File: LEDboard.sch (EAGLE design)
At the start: 312 parts, among them IC1 REG1117, Q1 MMUN2133LT1G, U1 IS31FL3741_QFN60, U2 IS31FL3741_QFN60, U3 ATSAMD21G-A, U4 TPS61090RSAR, U5 MCP73831T-2ACI/OT

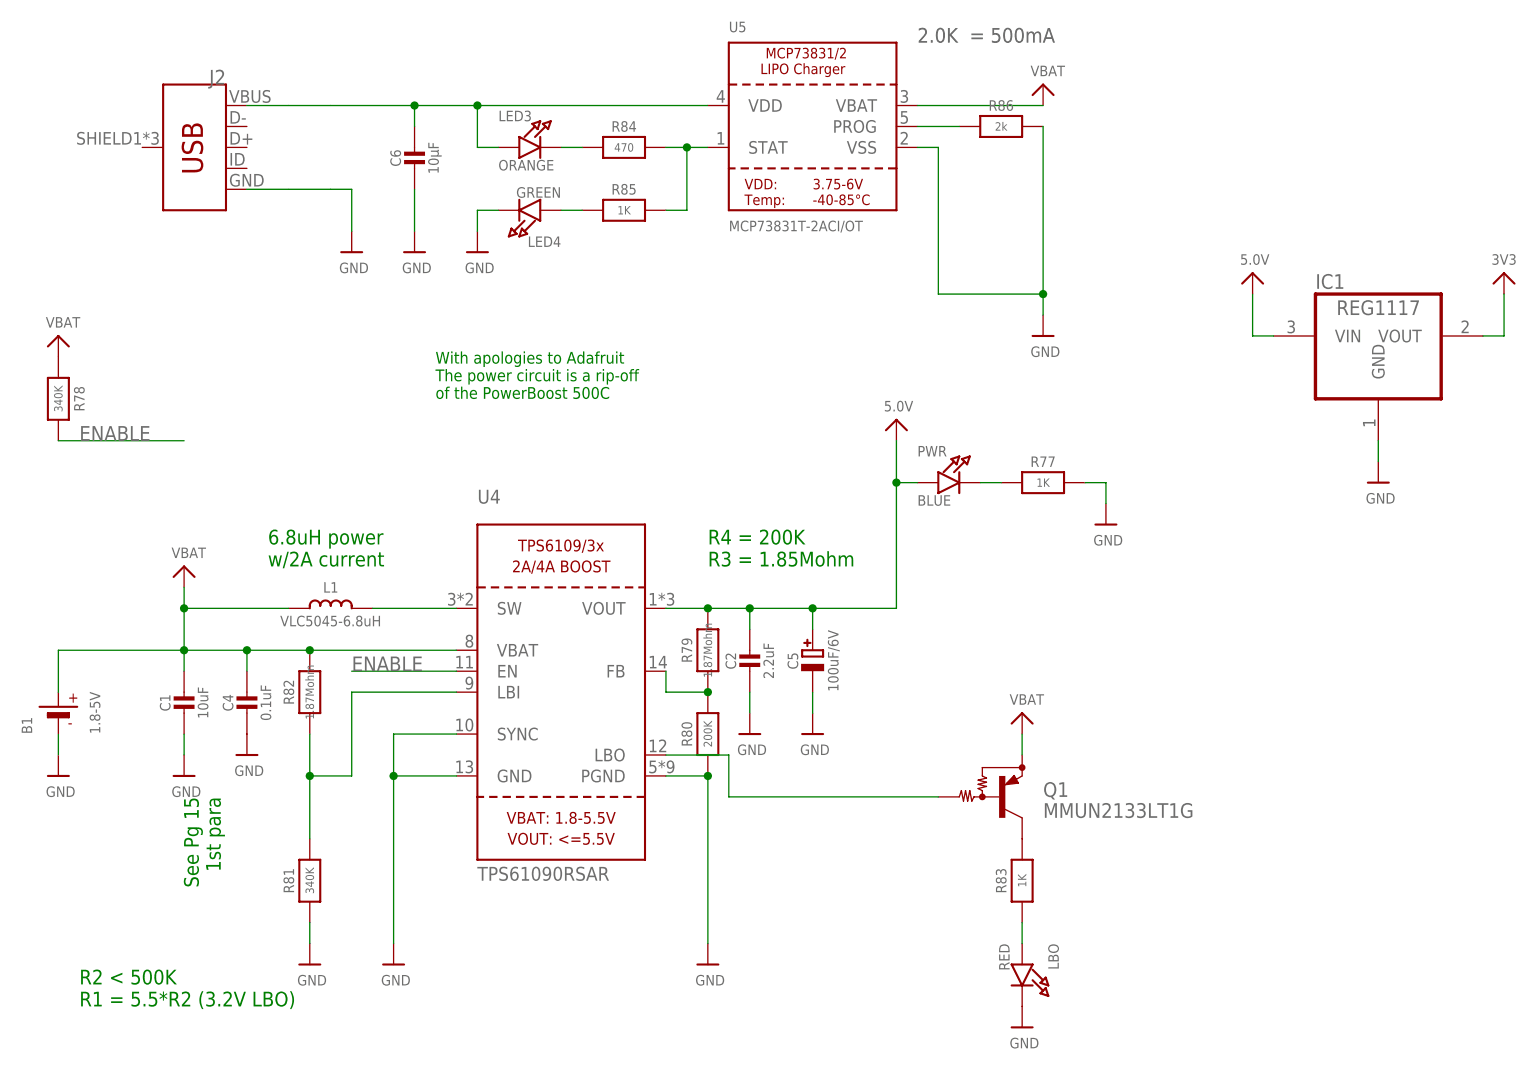
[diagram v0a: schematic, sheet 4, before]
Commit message: placed power
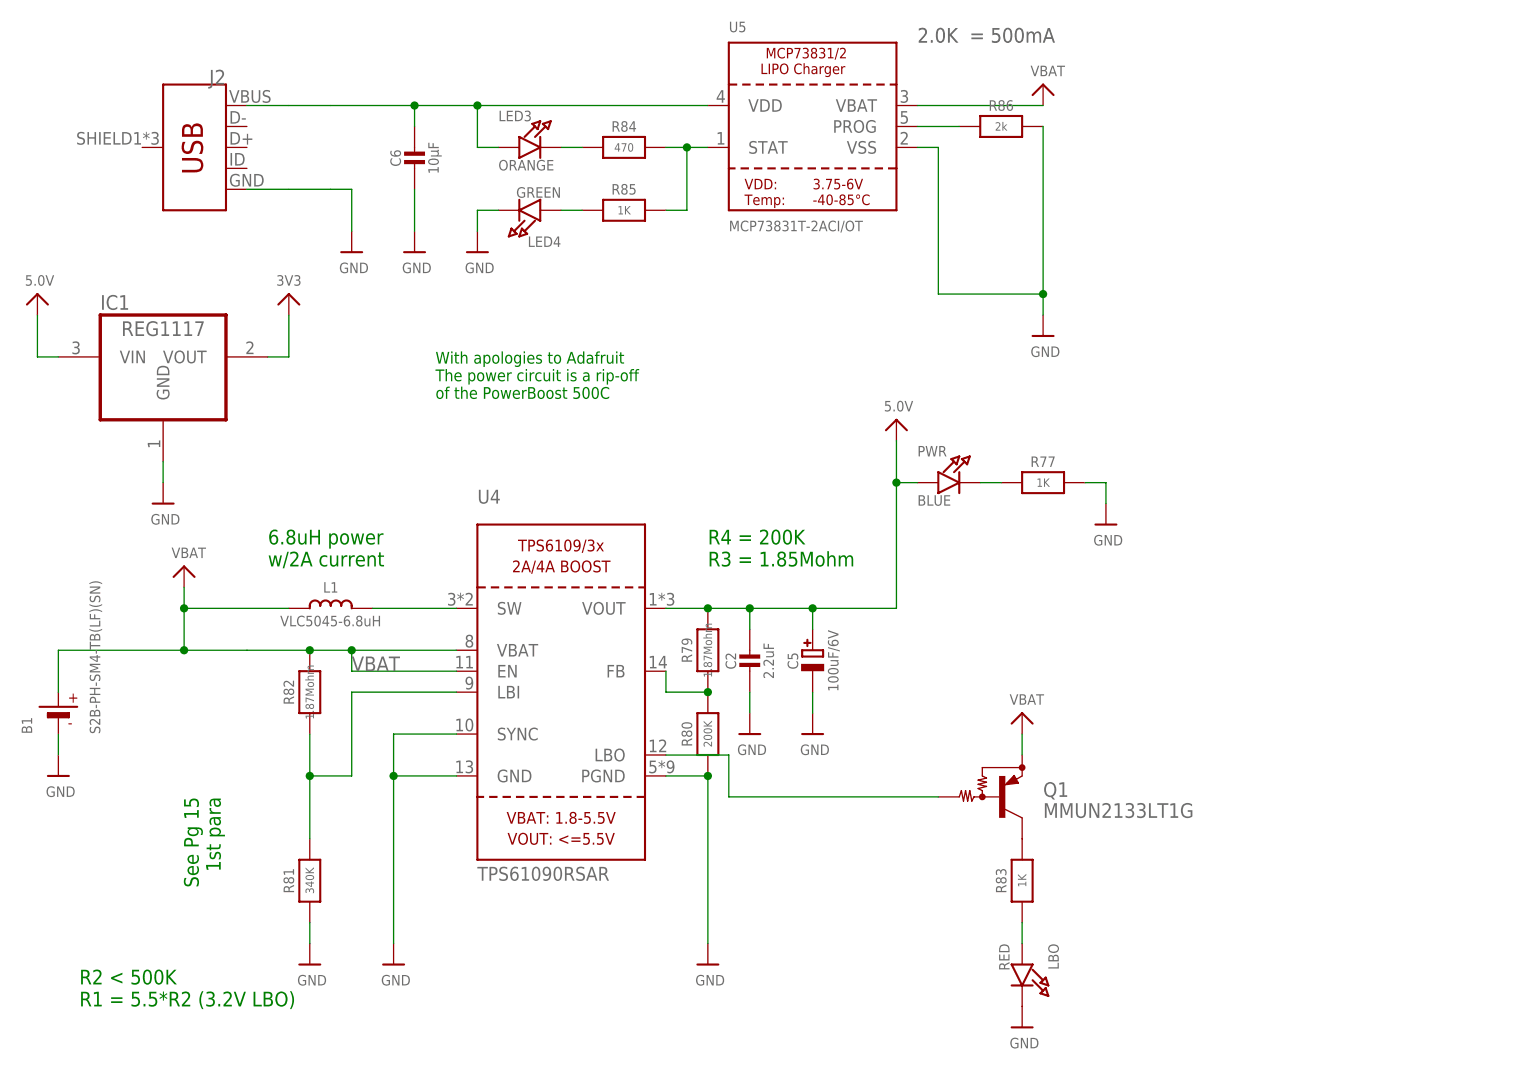
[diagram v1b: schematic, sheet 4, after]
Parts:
- removed C1: 10uF, microbuilder:CAP_CERAMIC0805-NOOUTLINE
- removed C4: 0.1uF, microbuilder:CAP_CERAMIC0805-NOOUTLINE
- removed R78: 340K, microbuilder:RESISTOR0805_NOOUTLINE
- B1: value 1.8-5V -> S2B-PH-SM4-TB(LF)(SN)
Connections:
- removed net ENABLE: R78.2, U4.EN
- net GND: no longer C1.2, C4.2
- net VBAT: now also U4.EN; no longer C1.1, C4.1, R78.1
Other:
- moved on the sheet: IC1
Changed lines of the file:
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@@
 <part name="R72" library="SparkFun-Resistors" library_urn="urn:adsk.eagle:library:532" deviceset="14KOHM" device="-0603-1/10W-1%" package3d_urn="urn:adsk.eagle:package:39650/1" value="20Ω"/>
 <part name="U3" library="SparkFun-IC-Microcontroller" library_urn="urn:adsk.eagle:library:525" deviceset="ATSAMD21G" device="-A" package3d_urn="urn:adsk.eagle:package:38963/1"/>
-<part name="FRAME1" library="microbuilder" deviceset="FRAME_A4" device=""/>
 <part name="U4" library="microbuilder" deviceset="VREG_TPS6103X" device="" value="TPS61090RSAR"/>
 <part name="L1" library="microbuilder" deviceset="INDUCTOR" device="TDK_VLC5045" value="VLC5045-6.8uH"/>
 <part name="U$1" library="microbuilder" deviceset="GND" device=""/>
 <part name="U$2" library="microbuilder" deviceset="GND" device=""/>
-<part name="C1" library="microbuilder" deviceset="CAP_CERAMIC" device="0805-NOOUTLINE" value="10uF"/>
-<part name="U$4" library="microbuilder" deviceset="GND" device=""/>
-<part name="B1" library="microbuilder" deviceset="BATTERY" device="" value="1.8-5V"/>
+<part name="B1" library="microbuilder" deviceset="BATTERY" device="" value="S2B-PH-SM4-TB(LF)(SN)"/>
 <part name="U$5" library="microbuilder" deviceset="GND" device=""/>
 <part name="C2" library="microbuilder" deviceset="CAP_CERAMIC" device="0805-NOOUTLINE" value="2.2uF"/>
@@
 <part name="PWR" library="microbuilder" deviceset="LED" device="0805_NOOUTLINE" value="BLUE"/>
 <part name="R77" library="microbuilder" deviceset="RESISTOR" device="0805_NOOUTLINE" value="1K"/>
-<part name="R78" library="microbuilder" deviceset="RESISTOR" device="0805_NOOUTLINE" value="340K"/>
-<part name="U$27" library="microbuilder" deviceset="VBAT" device=""/>
-<part name="U$24" library="microbuilder" deviceset="GND" device=""/>
-<part name="C4" library="microbuilder" deviceset="CAP_CERAMIC" device="0805-NOOUTLINE" value="0.1uF"/>
 <part name="R79" library="microbuilder" deviceset="RESISTOR" device="0805_NOOUTLINE" value="1.87Mohm"/>
 <part name="R80" library="microbuilder" deviceset="RESISTOR" device="0805_NOOUTLINE" value="200K"/>
@@
 <part name="U$33" library="microbuilder" deviceset="GND" device=""/>
 <part name="U$34" library="microbuilder" deviceset="VBAT" device=""/>
-<part name="U$23" library="microbuilder" deviceset="FRAME_A4_ADAFRUIT" device=""/>
 <part name="J2" library="SparkFun-Connectors" library_urn="urn:adsk.eagle:library:513" deviceset="USB_MICRO-B" device="_FEMALE-SMT" package3d_urn="urn:adsk.eagle:package:38238/1"/>
 <part name="IC1" library="burr-brown" library_urn="urn:adsk.eagle:library:111" deviceset="REG1117" device="" package3d_urn="urn:adsk.eagle:package:4940/1"/>
@@
 </plain>
 <instances>
-<instance part="FRAME1" gate="G$3" x="7.62" y="142.24"/>
 <instance part="U4" gate="G$1" x="83.82" y="58.42"/>
 <instance part="L1" gate="G$1" x="55.88" y="68.58"/>
 <instance part="U$1" gate="G$1" x="53.34" y="25.4"/>
 <instance part="U$2" gate="G$1" x="63.5" y="25.4"/>
-<instance part="C1" gate="G$1" x="38.1" y="55.88"/>
-<instance part="U$4" gate="G$1" x="38.1" y="48.26"/>
 <instance part="B1" gate="G$1" x="22.86" y="55.88" rot="R90"/>
 <instance part="U$5" gate="G$1" x="22.86" y="48.26"/>
@@
 <instance part="PWR" gate="G$1" x="132.08" y="83.82"/>
 <instance part="R77" gate="G$1" x="142.24" y="83.82"/>
-<instance part="R78" gate="G$1" x="22.86" y="93.98" rot="R270"/>
-<instance part="U$27" gate="G$1" x="22.86" y="101.6"/>
-<instance part="U$24" gate="G$1" x="45.72" y="50.8"/>
-<instance part="C4" gate="G$1" x="45.72" y="55.88"/>
 <instance part="R79" gate="G$1" x="101.6" y="63.5" rot="R90"/>
 <instance part="R80" gate="G$1" x="101.6" y="53.34" rot="R90"/>
@@
 <instance part="U$33" gate="G$1" x="73.66" y="111.76"/>
 <instance part="U$34" gate="G$1" x="142.24" y="132.08"/>
-<instance part="U$23" gate="G$1" x="2.54" y="2.54"/>
 <instance part="J2" gate="G$1" x="40.64" y="124.46" rot="MR0"/>
-<instance part="IC1" gate="G$1" x="182.88" y="101.6"/>
-<instance part="U$10" gate="G$1" x="182.88" y="83.82"/>
-<instance part="U$12" gate="G$1" x="167.64" y="109.22"/>
-<instance part="U$13" gate="G$1" x="198.12" y="109.22"/>
+<instance part="IC1" gate="G$1" x="35.56" y="99.06"/>
+<instance part="U$10" gate="G$1" x="35.56" y="81.28"/>
+<instance part="U$12" gate="G$1" x="20.32" y="106.68"/>
+<instance part="U$13" gate="G$1" x="50.8" y="106.68"/>
 </instances>
 <busses>
@@
 </segment>
 <segment>
-<pinref part="C1" gate="G$1" pin="2"/>
-<pinref part="U$4" gate="G$1" pin="GND"/>
-<wire x1="38.1" y1="53.34" x2="38.1" y2="50.8" width="0.1524" layer="91"/>
-</segment>
-<segment>
 <pinref part="B1" gate="G$1" pin="-"/>
 <pinref part="U$5" gate="G$1" pin="GND"/>
@@
 </segment>
 <segment>
-<pinref part="U$24" gate="G$1" pin="GND"/>
-<pinref part="C4" gate="G$1" pin="2"/>
-</segment>
-<segment>
 <pinref part="U4" gate="G$1" pin="PGND"/>
 <wire x1="96.52" y1="48.26" x2="101.6" y2="48.26" width="0.1524" layer="91"/>
@@
 </segment>
 <segment>
-<wire x1="182.88" y1="88.9" x2="182.88" y2="86.36" width="0.1524" layer="91"/>
+<wire x1="35.56" y1="86.36" x2="35.56" y2="83.82" width="0.1524" layer="91"/>
 <pinref part="U$10" gate="G$1" pin="GND"/>
 <pinref part="IC1" gate="G$1" pin="GND"/>
@@
 <segment>
 <pinref part="U$12" gate="G$1" pin="5.0V"/>
-<wire x1="167.64" y1="101.6" x2="167.64" y2="106.68" width="0.1524" layer="91"/>
+<wire x1="20.32" y1="99.06" x2="20.32" y2="104.14" width="0.1524" layer="91"/>
 <pinref part="IC1" gate="G$1" pin="VIN"/>
-<wire x1="170.18" y1="101.6" x2="167.64" y2="101.6" width="0.1524" layer="91"/>
+<wire x1="22.86" y1="99.06" x2="20.32" y2="99.06" width="0.1524" layer="91"/>
 </segment>
 </net>
 <net name="VBAT" class="0">
 <segment>
-<pinref part="R78" gate="G$1" pin="1"/>
-<pinref part="U$27" gate="G$1" pin="VBAT"/>
-</segment>
-<segment>
 <pinref part="U4" gate="G$1" pin="VBAT"/>
-<wire x1="71.12" y1="63.5" x2="53.34" y2="63.5" width="0.1524" layer="91"/>
+<wire x1="71.12" y1="63.5" x2="58.42" y2="63.5" width="0.1524" layer="91"/>
+<wire x1="58.42" y1="63.5" x2="53.34" y2="63.5" width="0.1524" layer="91"/>
 <wire x1="53.34" y1="63.5" x2="45.72" y2="63.5" width="0.1524" layer="91"/>
 <wire x1="45.72" y1="63.5" x2="38.1" y2="63.5" width="0.1524" layer="91"/>
-<pinref part="C1" gate="G$1" pin="1"/>
-<wire x1="38.1" y1="63.5" x2="38.1" y2="60.96" width="0.1524" layer="91"/>
 <pinref part="L1" gate="G$1" pin="1"/>
 <wire x1="50.8" y1="68.58" x2="38.1" y2="68.58" width="0.1524" layer="91"/>
 <wire x1="38.1" y1="68.58" x2="38.1" y2="63.5" width="0.1524" layer="91"/>
 <junction x="38.1" y="63.5"/>
-<wire x1="45.72" y1="60.96" x2="45.72" y2="63.5" width="0.1524" layer="91"/>
-<junction x="45.72" y="63.5"/>
 <pinref part="U$19" gate="G$1" pin="VBAT"/>
 <wire x1="38.1" y1="68.58" x2="38.1" y2="71.12" width="0.1524" layer="91"/>
 <junction x="38.1" y="68.58"/>
-<pinref part="C4" gate="G$1" pin="1"/>
 <pinref part="R82" gate="G$1" pin="2"/>
 <junction x="53.34" y="63.5"/>
@@
 <wire x1="22.86" y1="63.5" x2="22.86" y2="58.42" width="0.1524" layer="91"/>
 <wire x1="22.86" y1="63.5" x2="38.1" y2="63.5" width="0.1524" layer="91"/>
+<pinref part="U4" gate="G$1" pin="EN"/>
+<wire x1="71.12" y1="60.96" x2="58.42" y2="60.96" width="0.1524" layer="91"/>
+<label x="58.42" y="60.96" size="1.778" layer="95"/>
+<wire x1="58.42" y1="60.96" x2="58.42" y2="63.5" width="0.1524" layer="91"/>
+<junction x="58.42" y="63.5"/>
 </segment>
 <segment>
@@
 </segment>
 </net>
-<net name="ENABLE" class="0">
-<segment>
-<wire x1="38.1" y1="88.9" x2="22.86" y2="88.9" width="0.1524" layer="91"/>
-<label x="25.4" y="88.9" size="1.778" layer="95"/>
-<pinref part="R78" gate="G$1" pin="2"/>
-</segment>
-<segment>
-<pinref part="U4" gate="G$1" pin="EN"/>
-<wire x1="71.12" y1="60.96" x2="58.42" y2="60.96" width="0.1524" layer="91"/>
-<label x="58.42" y="60.96" size="1.778" layer="95"/>
-</segment>
-</net>
 <net name="N$76" class="0">
 <segment>
@@
 <segment>
 <pinref part="U$13" gate="G$1" pin="5.0V"/>
-<wire x1="198.12" y1="101.6" x2="198.12" y2="106.68" width="0.1524" layer="91"/>
+<wire x1="50.8" y1="99.06" x2="50.8" y2="104.14" width="0.1524" layer="91"/>
 <pinref part="IC1" gate="G$1" pin="VOUT"/>
-<wire x1="195.58" y1="101.6" x2="198.12" y2="101.6" width="0.1524" layer="91"/>
+<wire x1="48.26" y1="99.06" x2="50.8" y2="99.06" width="0.1524" layer="91"/>
 </segment>
 </net>

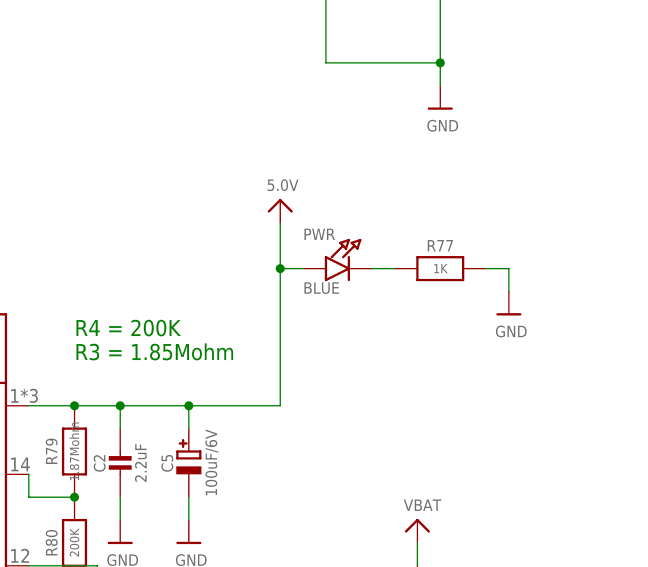
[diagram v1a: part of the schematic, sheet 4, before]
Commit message: dear fucking god
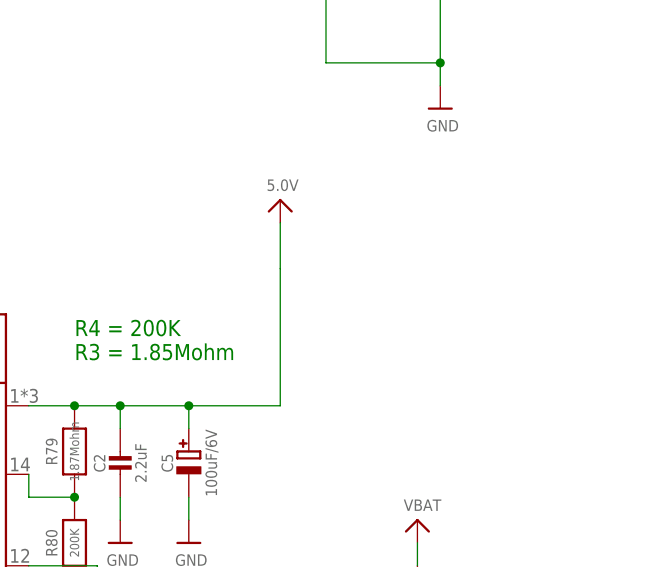
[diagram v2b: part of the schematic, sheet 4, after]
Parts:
- removed PWR: BLUE, microbuilder:LED0805_NOOUTLINE
- removed R77: 1K, microbuilder:RESISTOR0805_NOOUTLINE
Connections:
- removed net N$75: PWR.C, R77.1
- net 5.0V: no longer PWR.A
- net GND: no longer R77.2
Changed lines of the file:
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@@
 <part name="U$7" library="microbuilder" deviceset="5.0V" device=""/>
 <part name="U$19" library="microbuilder" deviceset="VBAT" device=""/>
-<part name="PWR" library="microbuilder" deviceset="LED" device="0805_NOOUTLINE" value="BLUE"/>
-<part name="R77" library="microbuilder" deviceset="RESISTOR" device="0805_NOOUTLINE" value="1K"/>
 <part name="R79" library="microbuilder" deviceset="RESISTOR" device="0805_NOOUTLINE" value="1.87Mohm"/>
 <part name="R80" library="microbuilder" deviceset="RESISTOR" device="0805_NOOUTLINE" value="200K"/>
@@
 <part name="U$6" library="microbuilder" deviceset="GND" device=""/>
 <part name="U$8" library="microbuilder" deviceset="GND" device=""/>
-<part name="U$14" library="microbuilder" deviceset="GND" device=""/>
 <part name="R81" library="microbuilder" deviceset="RESISTOR" device="0805_NOOUTLINE" value="340K"/>
 <part name="R82" library="microbuilder" deviceset="RESISTOR" device="0805_NOOUTLINE" value="1.87Mohm"/>
@@
 <instance part="U$7" gate="G$1" x="124.46" y="91.44"/>
 <instance part="U$19" gate="G$1" x="38.1" y="73.66"/>
-<instance part="PWR" gate="G$1" x="132.08" y="83.82"/>
-<instance part="R77" gate="G$1" x="142.24" y="83.82"/>
 <instance part="R79" gate="G$1" x="101.6" y="63.5" rot="R90"/>
 <instance part="R80" gate="G$1" x="101.6" y="53.34" rot="R90"/>
@@
 <instance part="U$6" gate="G$1" x="106.68" y="53.34"/>
 <instance part="U$8" gate="G$1" x="114.3" y="53.34"/>
-<instance part="U$14" gate="G$1" x="149.86" y="78.74"/>
 <instance part="R81" gate="G$1" x="53.34" y="35.56" rot="R90"/>
 <instance part="R82" gate="G$1" x="53.34" y="58.42" rot="R90"/>
@@
 </segment>
 <segment>
-<pinref part="R77" gate="G$1" pin="2"/>
-<wire x1="147.32" y1="83.82" x2="149.86" y2="83.82" width="0.1524" layer="91"/>
-<wire x1="149.86" y1="83.82" x2="149.86" y2="81.28" width="0.1524" layer="91"/>
-<pinref part="U$14" gate="G$1" pin="GND"/>
-</segment>
-<segment>
 <pinref part="U$1" gate="G$1" pin="GND"/>
 <pinref part="R81" gate="G$1" pin="1"/>
@@
 <wire x1="106.68" y1="66.04" x2="106.68" y2="68.58" width="0.1524" layer="91"/>
 <junction x="106.68" y="68.58"/>
-<pinref part="PWR" gate="G$1" pin="A"/>
-<wire x1="127" y1="83.82" x2="124.46" y2="83.82" width="0.1524" layer="91"/>
-<junction x="124.46" y="83.82"/>
 <wire x1="114.3" y1="68.58" x2="114.3" y2="66.04" width="0.1524" layer="91"/>
 <junction x="114.3" y="68.58"/>
@@
 </segment>
 </net>
-<net name="N$75" class="0">
-<segment>
-<pinref part="PWR" gate="G$1" pin="C"/>
-<pinref part="R77" gate="G$1" pin="1"/>
-<wire x1="134.62" y1="83.82" x2="137.16" y2="83.82" width="0.1524" layer="91"/>
-</segment>
-</net>
